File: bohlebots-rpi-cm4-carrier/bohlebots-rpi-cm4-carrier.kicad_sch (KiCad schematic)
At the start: 3 parts, among them K1 Kicker, T1 Taster_LED, U1 Compute_Module_4_Connectors

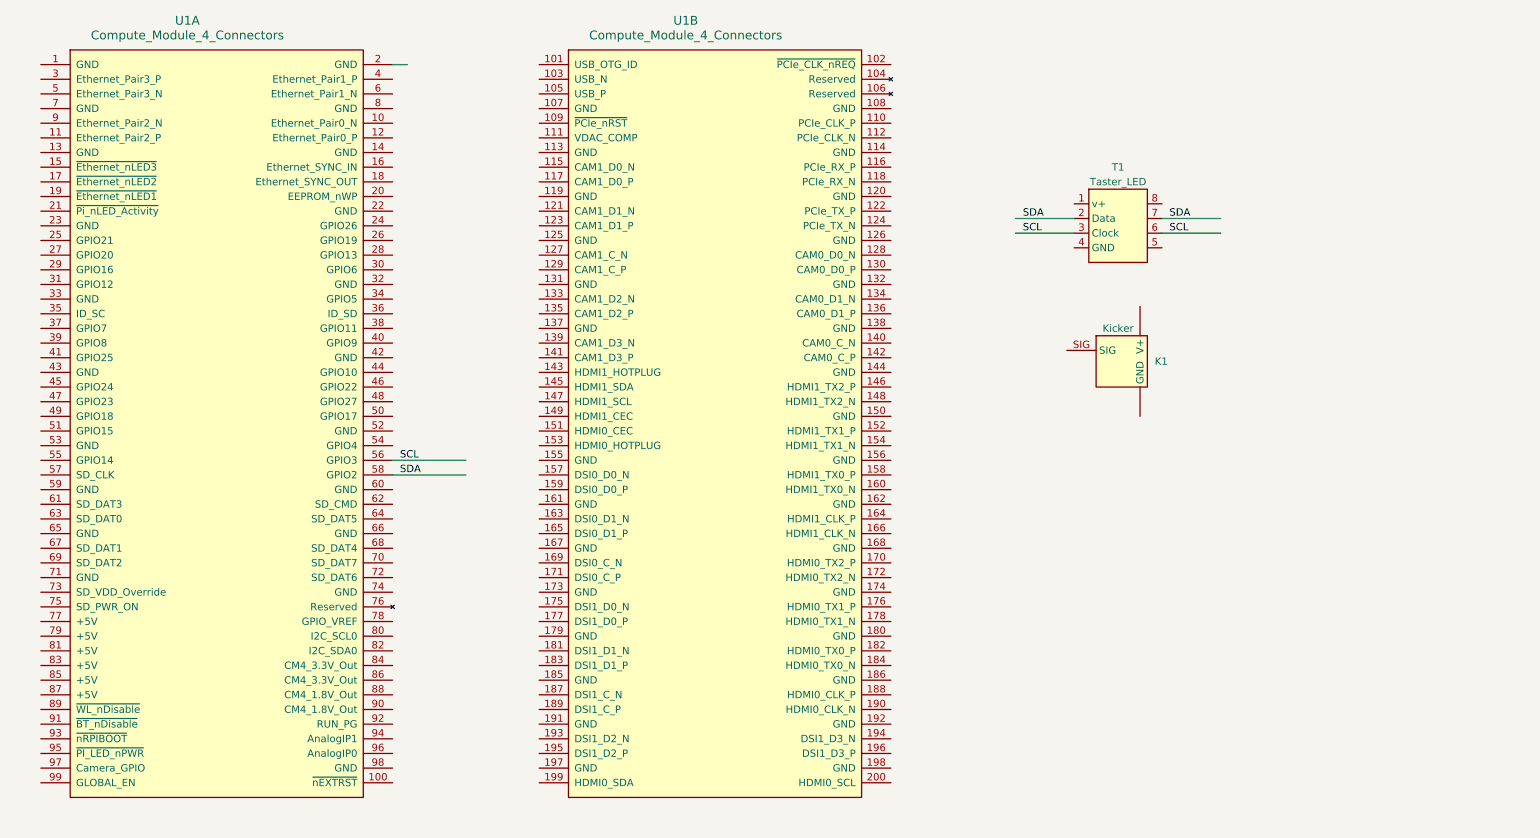
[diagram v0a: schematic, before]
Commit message: Schaltplan Update
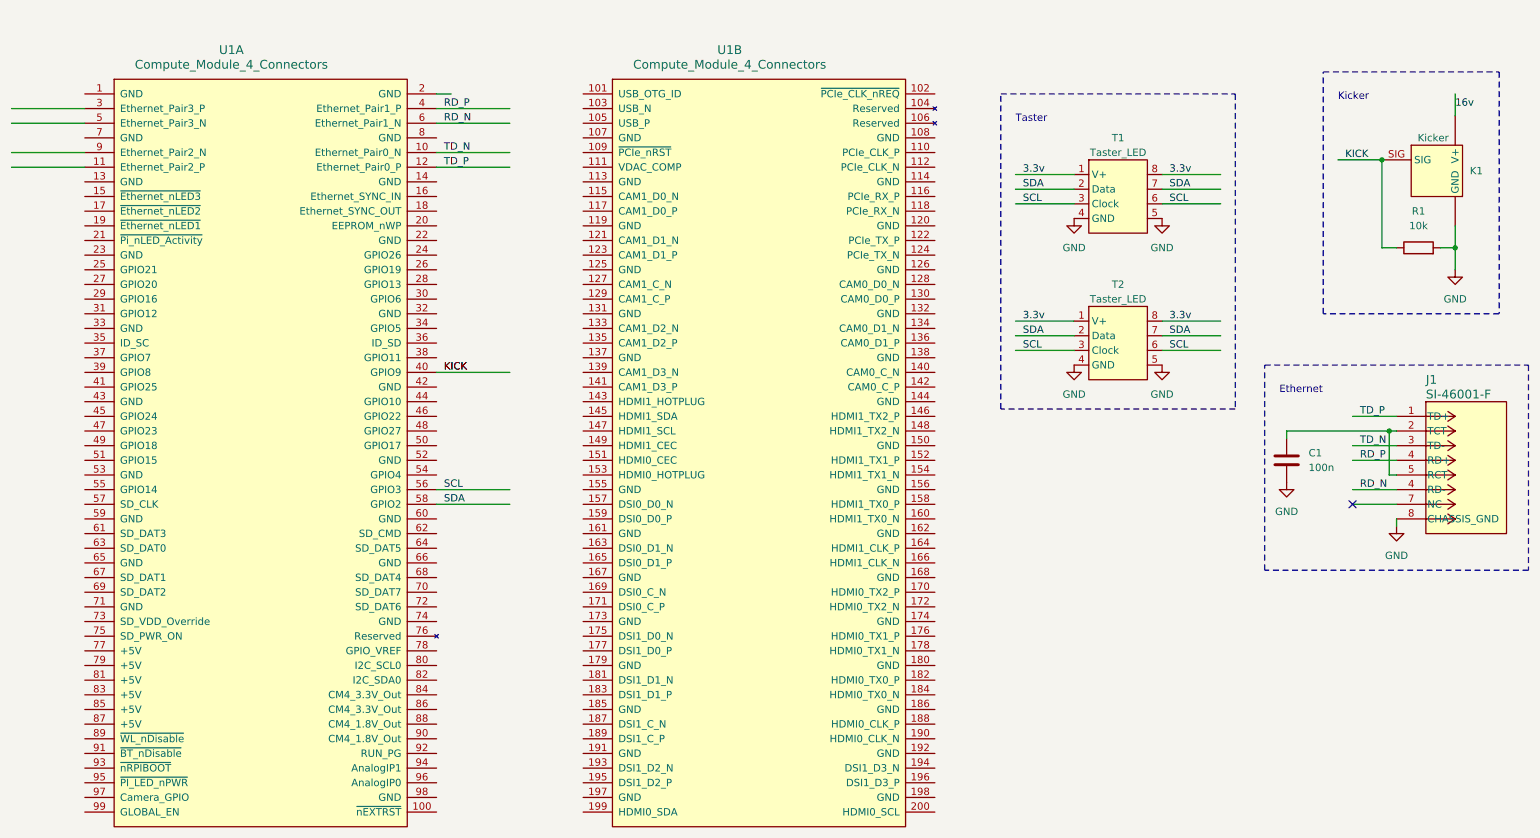
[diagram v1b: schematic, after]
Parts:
- added C1: 100n, Capacitor_THT:CP_Axial_L10.0mm_D4.5mm_P15.00mm_Horizontal, symbol Device:C
- added J1: SI-46001-F, SI_46001_F:CONN_46001-F_BEL, symbol SI_46001_F:SI-46001-F
- added R1: 10k, Resistor_THT:R_Array_SIP4, symbol Device:R
- added T2: Taster_LED, bohlebots:TASTER_LED, symbol bohlebots.lib:Taster_Led
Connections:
- net SCL: now also T2.3 (Clock), T2.6
- net SDA: now also T2.2 (Data), T2.7
- net 3.3v: now reaches T1.1 (V+)
- net 3.3v: now also T1.8, T2.1 (V+), T2.8
- net GND: now reaches T1.4 (GND)
- net GND: now also K1.GND1 (GND), K1.GND2 (GND), K1.GND3 (GND), K1.GND4 (GND), K1.GND5 (GND), K1.GND6 (GND), K1.GND7 (GND), K1.GND8 (GND), T1.5, C1.2, J1.8 (CHASSIS_GND), R1.2, T2.4 (GND), T2.5
- net TD_N: now reaches U1.10 (Ethernet_Pair0_N)
- net TD_N: now also J1.3 (TD-)
- net TD_P: now reaches U1.12 (Ethernet_Pair0_P)
- net TD_P: now also J1.1 (TD+)
- net RD_P: now reaches U1.4 (Ethernet_Pair1_P)
- net RD_P: now also J1.4 (RD-)
- net KICK: now reaches U1.40 (GPIO9)
- net KICK: now also K1.SIG, R1.1
- net RD_N: now reaches U1.6 (Ethernet_Pair1_N)
- net RD_N: now also J1.4 (RD-)
- net 16v: now reaches K1.V+1 (V+), K1.V+2 (V+), K1.V+3 (V+)
- new net: C1.1, J1.2 (TCT), J1.5 (RCT)
- no-connect marks 0 -> 1
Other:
- note added: "Ethernet"
- note added: "Kicker"
- note added: "Taster"
- moved on the sheet: K1, T1, U1A, U1B
